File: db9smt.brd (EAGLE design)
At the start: 15 x 30.7 mm, 21 parts, among them CON1 PADONPRINT, CON2 PADONPRINT, CON3 PADONPRINT, CON4 PADONPRINT, CON5 PADONPRINT, CON6 PADONPRINT, CON7 PADONPRINT, CON8 PADONPRINT, CON9 PADONPRINT

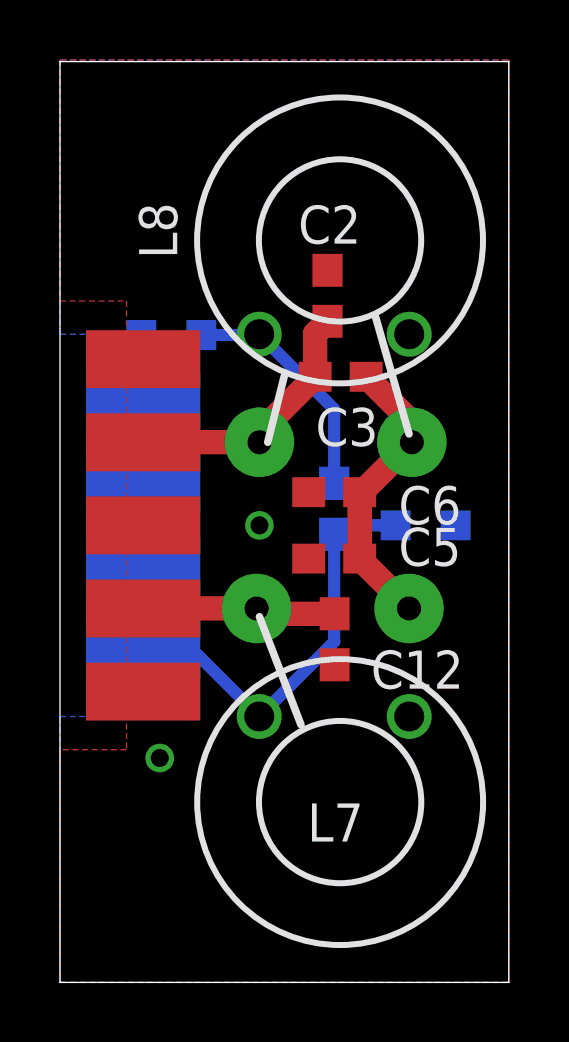
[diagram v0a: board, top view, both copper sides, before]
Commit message: Minor fix DB9SMT
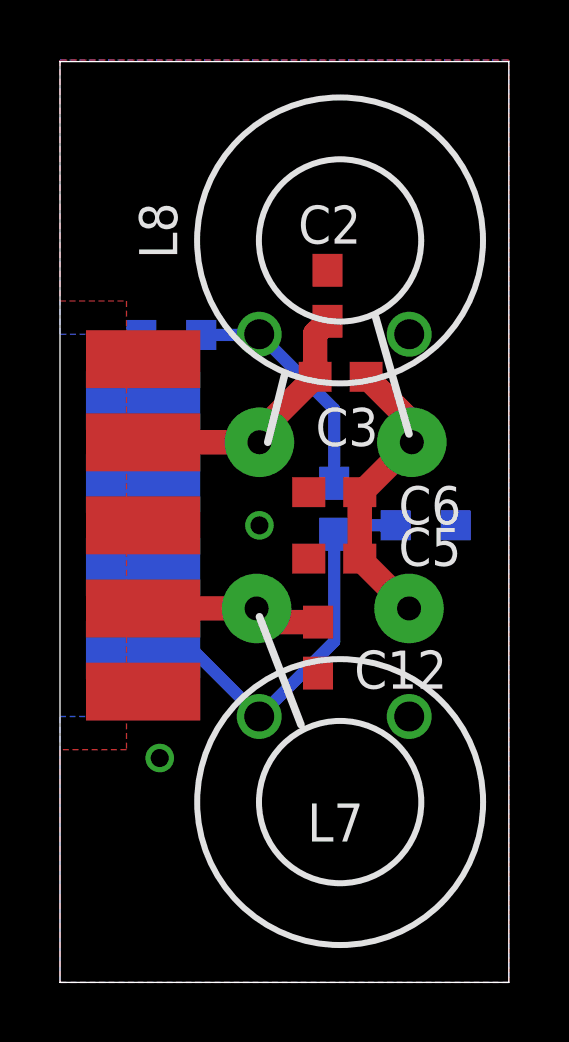
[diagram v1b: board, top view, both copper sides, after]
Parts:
- moved C12 0.62 mm to (8.60, 11.2)
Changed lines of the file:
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@@
 <attribute name="SPICEPREFIX" value="C" x="8.917" y="22.886" size="1.778" layer="27" rot="R90" display="off"/>
 </element>
-<element name="C12" library="eagle-ltspice" package="C0603" value="150p" x="9.156" y="11.437" smashed="yes" rot="R270">
-<attribute name="NAME" x="10.365" y="9.791" size="1.27" layer="25"/>
-<attribute name="SPICEMODEL" value="NONE" x="9.156" y="11.437" size="1.778" layer="27" rot="R270" display="off"/>
-<attribute name="SPICEPREFIX" value="C" x="9.156" y="11.437" size="1.778" layer="27" rot="R270" display="off"/>
+<element name="C12" library="eagle-ltspice" package="C0603" value="150p" x="8.602" y="11.16" smashed="yes" rot="R270">
+<attribute name="NAME" x="9.811" y="9.791" size="1.27" layer="25"/>
+<attribute name="SPICEMODEL" value="NONE" x="8.602" y="11.16" size="1.778" layer="27" rot="R270" display="off"/>
+<attribute name="SPICEPREFIX" value="C" x="8.602" y="11.16" size="1.778" layer="27" rot="R270" display="off"/>
 </element>
 <element name="C6" library="eagle-ltspice" package="C0603" value="330p" x="9.141" y="16.343" smashed="yes" rot="R180">
@@
 <contactref element="CON5" pad="P$1"/>
 <contactref element="CON1" pad="P$1"/>
-<wire x1="9.156" y1="10.587" x2="8.291" y2="14.127" width="0" layer="19" extent="1-1"/>
 </signal>
 <signal name="N$2">
@@
 <wire x1="6.554" y1="12.465" x2="6.653" y2="12.564" width="0.8128" layer="1"/>
 <wire x1="6.554" y1="12.465" x2="6.732" y2="12.287" width="0.8128" layer="1"/>
-<wire x1="6.732" y1="12.287" x2="9.156" y2="12.287" width="0.8128" layer="1"/>
+<wire x1="6.554" y1="12.465" x2="7.009" y2="12.01" width="0.8128" layer="1"/>
+<wire x1="7.009" y1="12.01" x2="8.602" y2="12.01" width="0.8128" layer="1"/>
 </signal>
 <signal name="N$6">
